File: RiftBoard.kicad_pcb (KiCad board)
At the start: 2 copper layers, 21 x 51.2 mm, 41 parts, among them J1 USB_C_Receptacle_USB2.0_16P, J2 Conn_01x20, J3 Conn_01x20, J4 Conn_01x03, SW1 SW_Push, SW2 SW_Push, U1 RP2040, U2 MCP1700x-330xxTT, U3 W25Q16JVUXIQ TR, Y1 12MHz

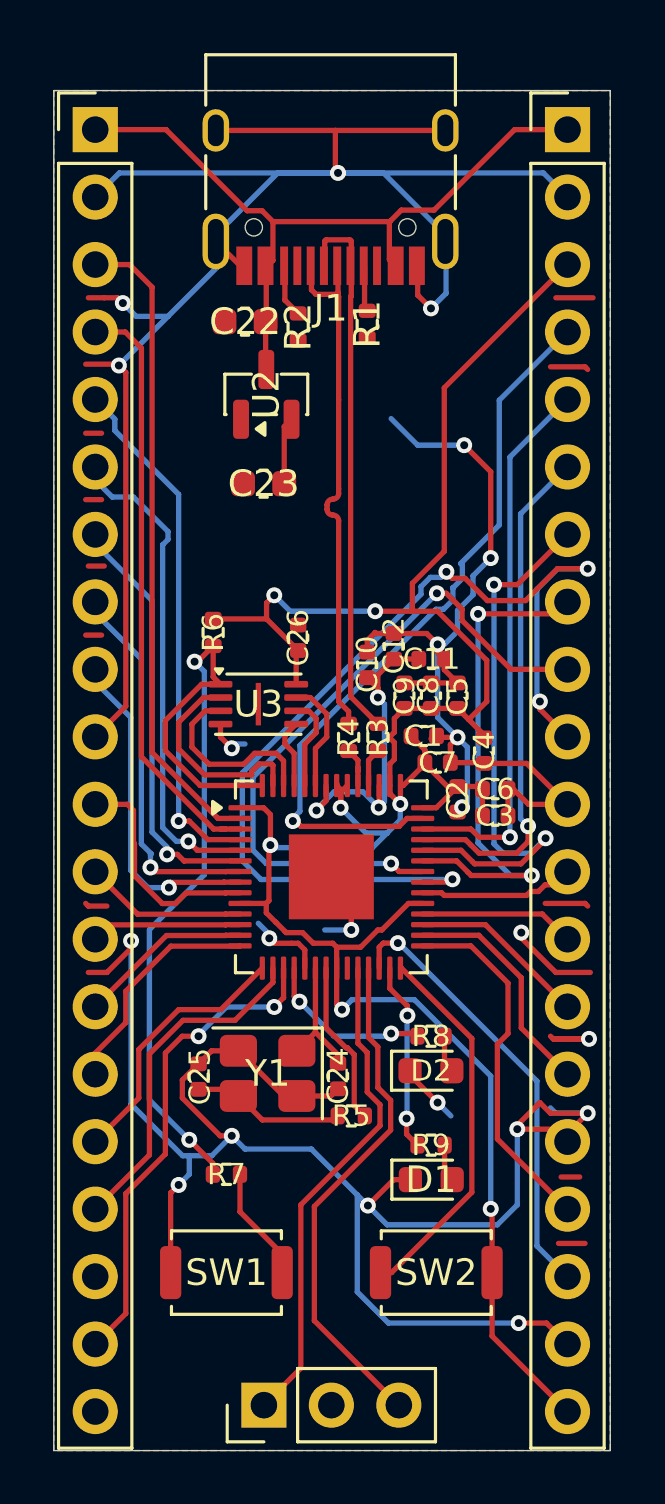
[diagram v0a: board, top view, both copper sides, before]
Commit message: Hopefully final fix
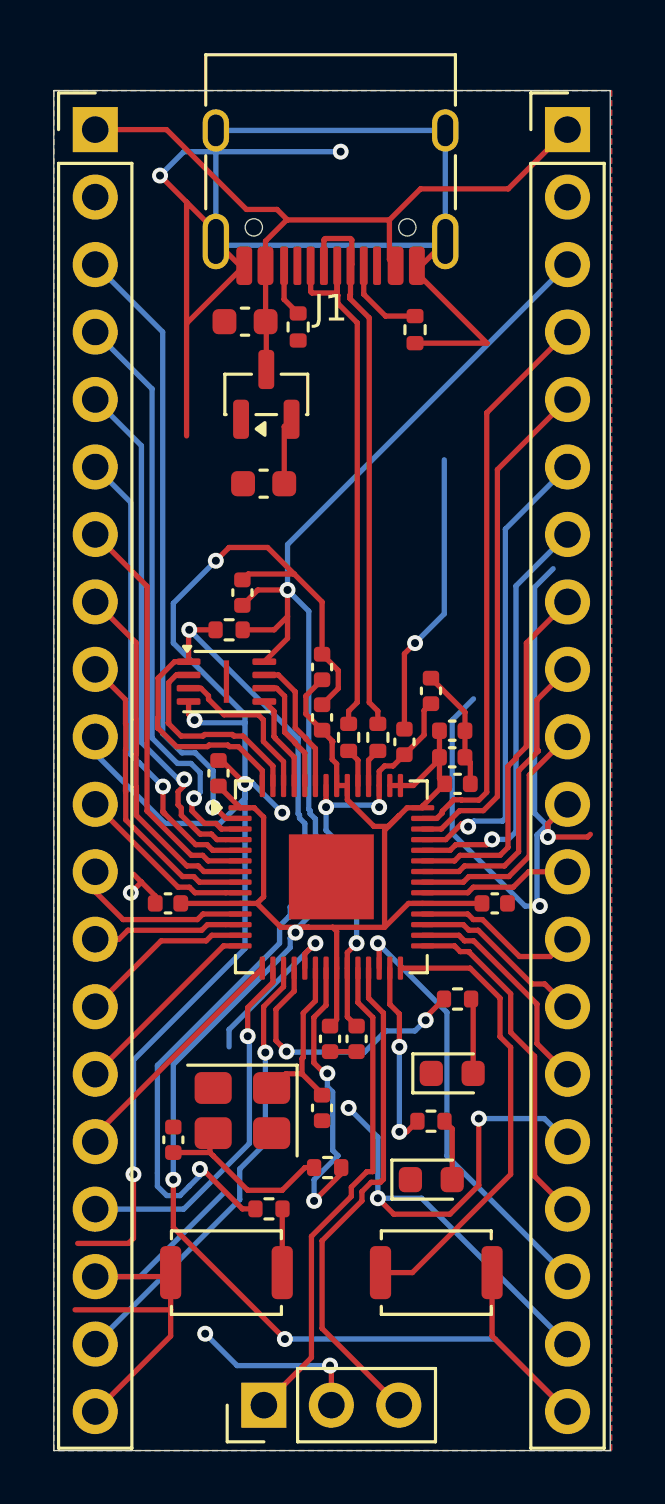
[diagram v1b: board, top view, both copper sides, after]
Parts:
- moved C11 14.6 mm to (105.2, 106.1), turned to -90 degrees
- moved C5 13.8 mm to (104.2, 106.1), turned to -90 degrees
- moved C6 13.0 mm to (98.1, 101.0), turned to 180 degrees
- moved C7 8.26 mm to (100.0, 96.1), turned to 90 degrees
- moved C4 5.76 mm to (110.4, 101.0), turned to 0 degrees
- moved C8 4.18 mm to (103.9, 94.0)
- moved C9 3.28 mm to (103.9, 92.1)
- moved C10 3.22 mm to (107.0, 94.9)
- moved C26 2.70 mm to (100.9, 89.3)
- moved C25 2.56 mm to (98.3, 109.9)
- moved C12 2.19 mm to (108.0, 93.0)
- moved R5 2.14 mm to (104.1, 110.9)
- moved R7 2.06 mm to (101.9, 112.5)
- moved C3 1.86 mm to (109.0, 96.5)
- moved R1 1.81 mm to (107.4, 79.4)
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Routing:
- net GPIO23: track 38.2 -> 9.51 mm, vias 4 -> 0
- net +3V3: track 94.8 -> 115.9 mm, vias 7 -> 4
- net GND: track 200.0 -> 217.5 mm, vias 22 -> 17
- net GPIO24: track 26.1 -> 11.6 mm, vias 2 -> 0
- net QSPI_SS: track 31.8 -> 40.8 mm
- net GPIO29/ADC3: track 28.0 -> 21.5 mm, vias 1 -> 0
- net GPIO25: track 19.4 -> 13.6 mm, vias 2 -> 0
- net GPIO26/ADC0: track 21.1 -> 15.8 mm, vias 2 -> 1
- net XOUT: track 6.20 -> 11.4 mm, vias 0 -> 2
- net +1V1: track 12.7 -> 16.8 mm
- net Net-(U1-GPIO15): track 6.50 -> 10.4 mm
- net GPIO17: track 14.3 -> 17.4 mm
- net GPIO28/ADC2: track 21.6 -> 19.4 mm, vias 1 -> 0
- net GPIO27/ADC1: track 19.7 -> 17.7 mm
- net Net-(R7-Pad1): track 4.36 -> 2.40 mm
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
